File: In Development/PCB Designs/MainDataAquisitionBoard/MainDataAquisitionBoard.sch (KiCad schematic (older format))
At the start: 21 parts, among them J1 Conn_01x08, J10 3v3, J11 TopR, J12 TopL, J13 BottomR, J14 BottomL, J15 RTC, J16 XbeeL, J17 XbeeR, J2 Conn_01x08, J3 GND, J4 1x24, J5 Teensy 3.6L, J6 Teensy 3.6R, J7 1x24, J8 5V, J9 Conn_01x04

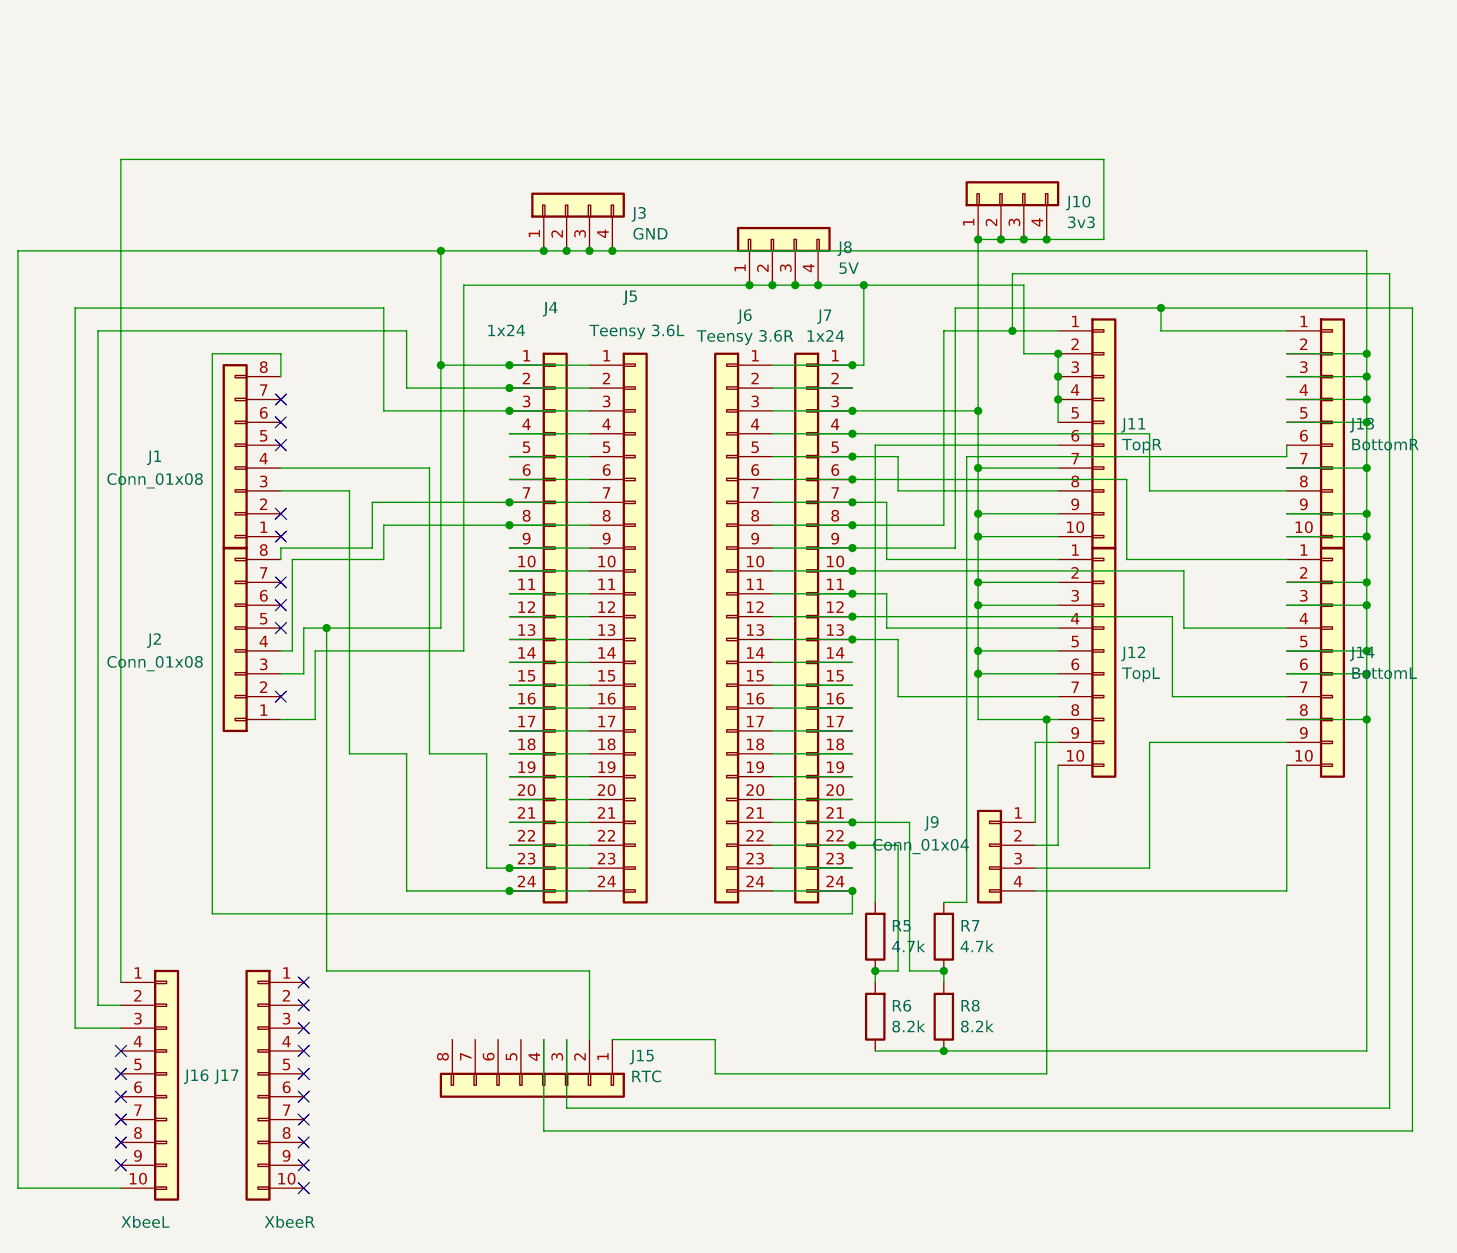
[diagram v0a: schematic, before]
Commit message: Finished DAQ board and ready for initial production
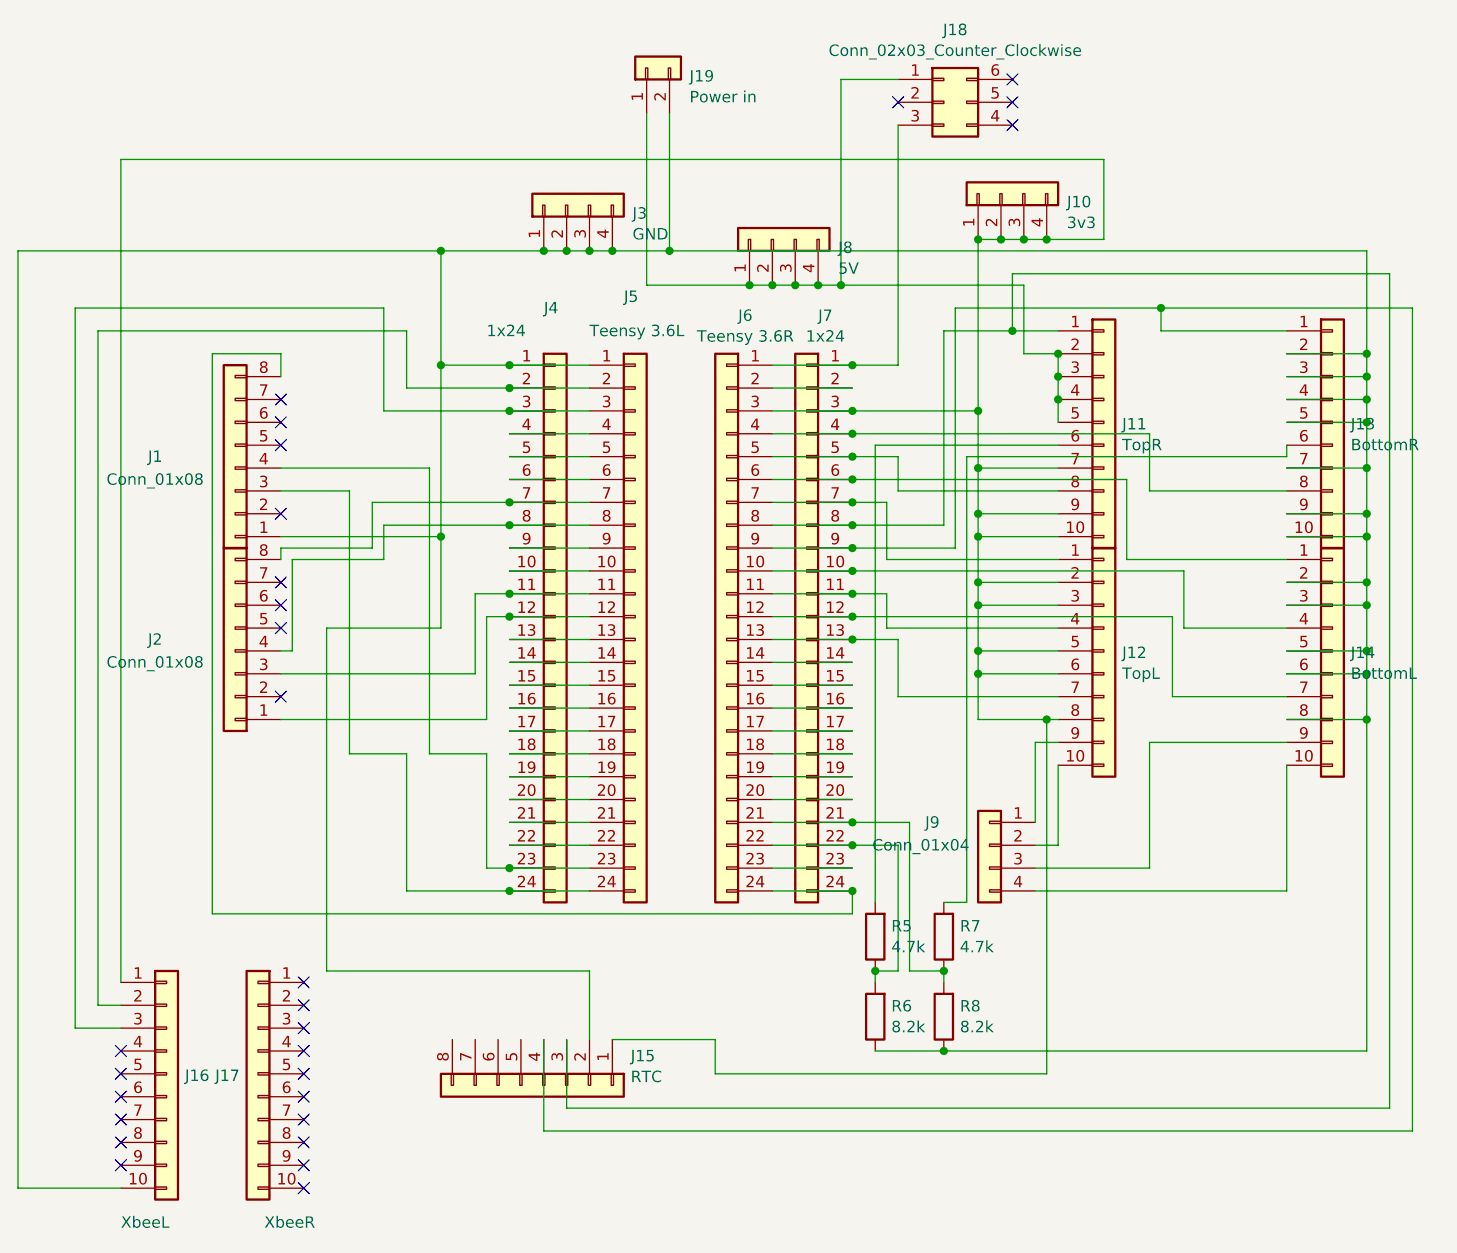
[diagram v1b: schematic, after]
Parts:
- added J18: Conn_02x03_Counter_Clockwise, Connector_PinHeader_2.54mm:PinHeader_2x03_P2.54mm_Vertical, symbol Connector_Generic:Conn_02x03_Counter_Clockwise
- added J19: Power in, CustomKiCADLibrary:PinHeader_1x02_P5.08mm_Vertical, symbol Connector_Generic:Conn_01x02
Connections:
- net at J13.10 (Pin_10), J13.2 (Pin_2), J13.3 (Pin_3)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: now also J1.1 (Pin_1), J19.2 (Pin_2); no longer J2.3 (Pin_3)
- net at J4.11 (Pin_11), J5.11 (Pin_11): now also J2.3 (Pin_3)
- net at J4.12 (Pin_12), J5.12 (Pin_12): now also J2.1 (Pin_1)
- net at J11.2 (Pin_2), J11.3 (Pin_3), J11.4 (Pin_4)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: now also J18.1 (Pin_1), J19.1 (Pin_1); no longer J2.1 (Pin_1), J6.1 (Pin_1), J7.1 (Pin_1)
- new net: J18.3 (Pin_3), J6.1 (Pin_1), J7.1 (Pin_1)
- no-connect marks 25 -> 28
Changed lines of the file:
@@
 $EndComp
-Wire Wire Line
-	4250 4200 4250 2600
-Wire Wire Line
-	6000 2600 6000 2950
 Wire Wire Line
 	5600 2950 5950 2950
 Connection ~ 5950 2950
 Wire Wire Line
-	5950 2950 6000 2950
-Wire Wire Line
-	3550 4100 3650 4100
-Wire Wire Line
 	4150 2950 4450 2950
 Connection ~ 4450 2950
@@
 Connection ~ 4450 3550
 Wire Wire Line
-	4100 4650 4350 4650
-Wire Wire Line
 	4350 4650 4350 5150
 Wire Wire Line
@@
 	4450 5150 4800 5150
 Wire Wire Line
-	3750 4650 4000 4650
-Wire Wire Line
-	4000 4650 4000 5250
-Wire Wire Line
 	4000 5250 4450 5250
 Connection ~ 4450 5250
-Connection ~ 3650 4100
-Wire Wire Line
-	3650 4100 4150 4100
-Wire Wire Line
-	4150 2950 4150 4100
-Wire Wire Line
-	6000 2600 6700 2600
 Wire Wire Line
 	6700 2600 6700 2900
 Wire Wire Line
 	6700 2900 6850 2900
-Connection ~ 6000 2600
 Wire Wire Line
 	6850 2900 6850 3000
@@
 Wire Wire Line
 	8200 2900 7850 2900
-Connection ~ 4150 2950
 Wire Wire Line
 	8200 4500 7850 4500
@@
 $EndComp
 Wire Wire Line
-	4900 2450 8200 2450
-Wire Wire Line
 	4600 2450 4700 2450
 Connection ~ 4600 2450
@@
 Wire Wire Line
 	4800 2450 4900 2450
-Wire Wire Line
-	5800 2600 6000 2600
 $Comp
 L Connector_Generic:Conn_01x04 J8
@@
 $EndComp
 Wire Wire Line
-	4250 2600 5500 2600
-Wire Wire Line
 	5500 2600 5600 2600
-Connection ~ 5500 2600
 Connection ~ 5800 2600
 Connection ~ 5600 2600
@@
 	3750 3500 3450 3500
 Wire Wire Line
-	4250 4200 3600 4200
-Wire Wire Line
-	3600 4200 3600 4500
-Wire Wire Line
-	3600 4500 3450 4500
-Wire Wire Line
-	3550 4100 3550 4300
-Wire Wire Line
-	3550 4300 3450 4300
-Wire Wire Line
 	3500 3800 3500 4200
 Wire Wire Line
 	3500 4200 3450 4200
 Wire Wire Line
-	3500 3800 3900 3800
-Wire Wire Line
 	3450 3750 3450 3800
 Wire Wire Line
@@
 Wire Wire Line
 	3450 3750 3850 3750
-NoConn ~ 3450 3700
 Wire Wire Line
 	6050 3300 6050 5300
@@
 	4600 6300 4600 5900
 Connection ~ 7300 2700
-Wire Wire Line
-	4100 3400 4100 4650
-Wire Wire Line
-	3750 3500 3750 4650
-Wire Wire Line
-	3650 4100 3650 5600
 $Comp
 L Connector_Generic:Conn_01x10 J16
@@
 Wire Wire Line
 	4450 3150 4800 3150
+$Comp
+L Connector_Generic:Conn_02x03_Counter_Clockwise J18
+U 1 1 5E28BDCC
+P 6350 1800
+F 0 "J18" H 6400 2117 50  0000 C CNN
+F 1 "Conn_02x03_Counter_Clockwise" H 6400 2026 50  0000 C CNN
+F 2 "Connector_PinHeader_2.54mm:PinHeader_2x03_P2.54mm_Vertical" H 6350 1800 50  0001 C CNN
+F 3 "~" H 6350 1800 50  0001 C CNN
+	1    6350 1800
+	1    0    0    -1
+$EndComp
+Wire Wire Line
+	5800 2600 5900 2600
+Wire Wire Line
+	5900 2600 5900 1700
+Wire Wire Line
+	5900 1700 6150 1700
+Connection ~ 5900 2600
+Wire Wire Line
+	5900 2600 6700 2600
+Wire Wire Line
+	6150 1900 6150 2950
+Wire Wire Line
+	5950 2950 6150 2950
+NoConn ~ 6150 1800
+NoConn ~ 6650 1700
+NoConn ~ 6650 1800
+NoConn ~ 6650 1900
+Connection ~ 4150 2950
+Wire Wire Line
+	3500 3800 3900 3800
+Wire Wire Line
+	3650 4100 3650 5600
+Wire Wire Line
+	3750 3500 3750 4650
+Wire Wire Line
+	4100 3400 4100 4650
+Wire Wire Line
+	4150 2950 4150 3700
+Wire Wire Line
+	3650 4100 4150 4100
+Wire Wire Line
+	4000 4650 4000 5250
+Wire Wire Line
+	3750 4650 4000 4650
+Wire Wire Line
+	4100 4650 4350 4650
+Wire Wire Line
+	3450 3700 4150 3700
+Connection ~ 4150 3700
+Wire Wire Line
+	4150 3700 4150 4100
+Wire Wire Line
+	3450 4300 4300 4300
+Wire Wire Line
+	4300 4300 4300 3950
+Wire Wire Line
+	4300 3950 4450 3950
+Connection ~ 4450 3950
+Wire Wire Line
+	3450 4500 4350 4500
+Wire Wire Line
+	4350 4500 4350 4050
+Wire Wire Line
+	4350 4050 4450 4050
+Connection ~ 4450 4050
+$Comp
+L Connector_Generic:Conn_01x02 J19
+U 1 1 5E3C057F
+P 5050 1650
+F 0 "J19" V 5014 1462 50  0000 R CNN
+F 1 "Power in" V 4923 1462 50  0000 R CNN
+F 2 "CustomKiCADLibrary:PinHeader_1x02_P5.08mm_Vertical" H 5050 1650 50  0001 C CNN
+F 3 "~" H 5050 1650 50  0001 C CNN
+	1    5050 1650
+	0    -1   -1   0
+$EndComp
+Wire Wire Line
+	5050 1850 5050 2600
+Wire Wire Line
+	5050 2600 5500 2600
+Connection ~ 5500 2600
+Wire Wire Line
+	5150 1850 5150 2450
+Wire Wire Line
+	4900 2450 5150 2450
+Connection ~ 5150 2450
+Wire Wire Line
+	5150 2450 8200 2450
 $EndSCHEMATC
